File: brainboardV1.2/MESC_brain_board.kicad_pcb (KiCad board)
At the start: 4 copper layers, 64 x 84.5 mm, 52 parts, among them J1 Conn_01x18, J12 Conn_01x03, J13 Conn_01x03, J14 SERIAL1, J15 Conn_01x03, J21 Conn_01x07, J22 Conn_01x01, J24 Conn_01x01, J25 Conn_01x01, Q1 my_BC337, U1 TJA1050T/CM,118, U11 ESP32-WROOM-32D, U2 Teensy4.0, U21 LD1117S18TR_SOT223, U24 12_DCDC_5

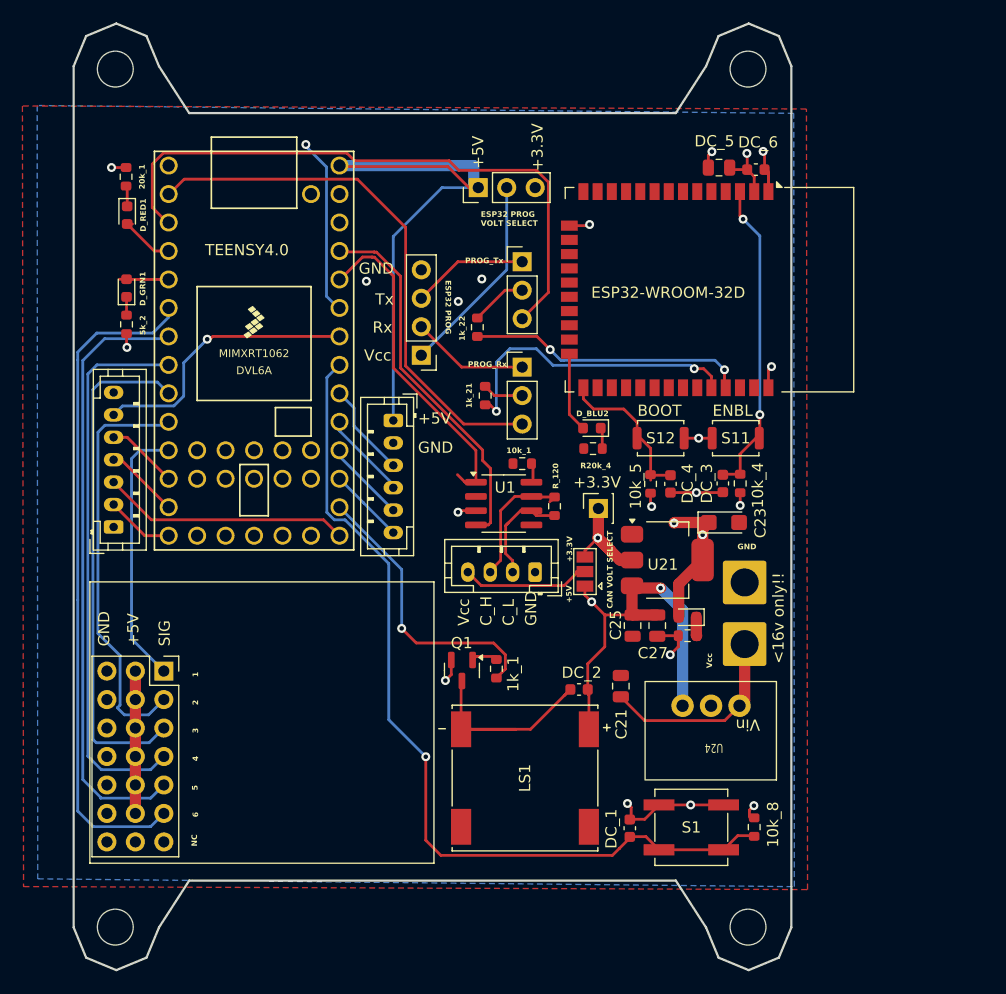
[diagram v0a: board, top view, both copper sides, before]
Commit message: documentation stuff
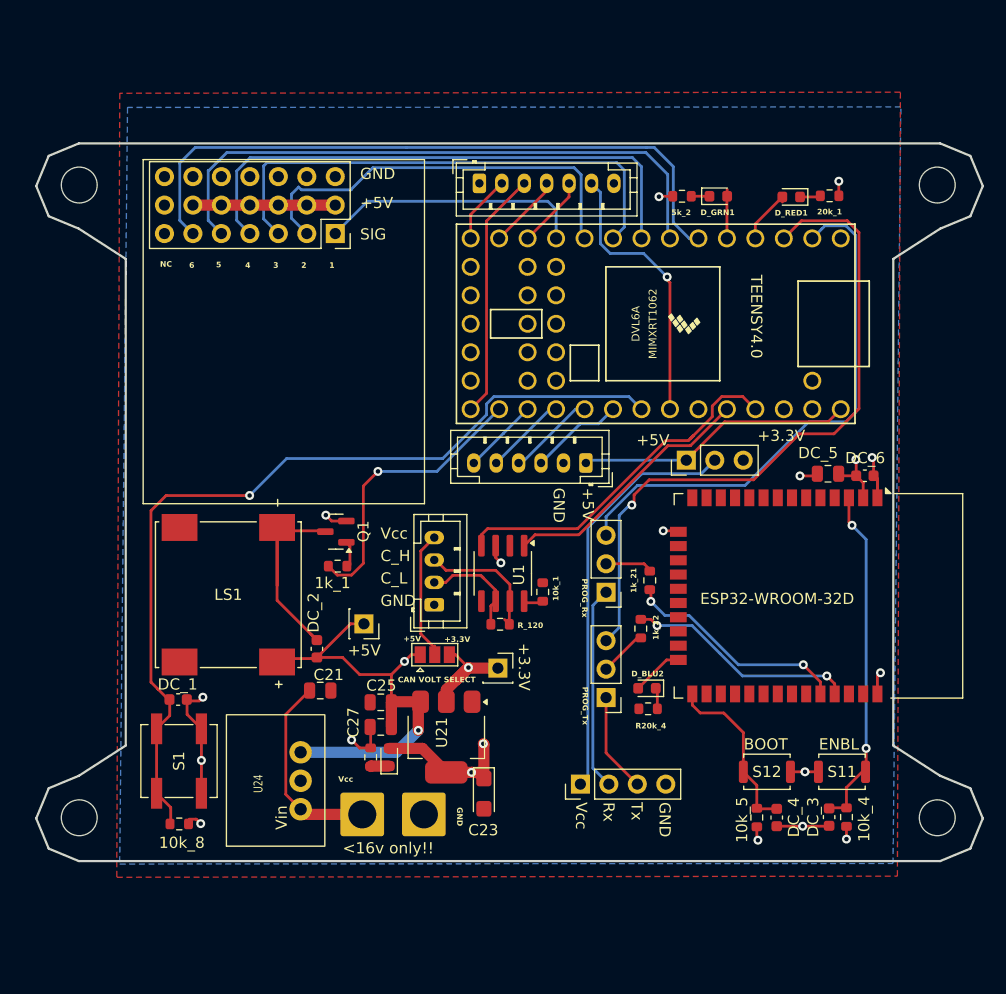
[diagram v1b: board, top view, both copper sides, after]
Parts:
- added J23: Conn_01x01, Connector_PinSocket_2.54mm:PinSocket_1x01_P2.54mm_Vertical, F.Cu at (45.5, 62.8)
- moved REF** 74.1 mm to (96.7, 23.7), turned to -90 degrees
- moved REF** 68.9 mm to (96.7, 80.1), turned to -90 degrees
- moved REF** 66.3 mm to (20.1, 23.7), turned to -90 degrees
- moved 20k_1 62.8 mm to (87.1, 24.7), turned to 180 degrees
- moved REF** 60.5 mm to (20.1, 80.1), turned to -90 degrees
- moved D_RED1 59.3 mm to (83.7, 24.8), turned to 180 degrees
- moved D_GRN1 53.4 mm to (77.1, 24.7), turned to 0 degrees
- moved 10k_8 51.3 mm to (29.1, 80.7), turned to 0 degrees
- moved 5k_2 50.9 mm to (73.9, 24.7), turned to 0 degrees
- moved S1 46.1 mm to (29.0, 75.1), turned to -90 degrees
- moved J21 44.8 mm to (55.8, 23.5), turned to 0 degrees
- moved J1 41.9 mm to (43.0, 28.0), turned to -90 degrees
- moved DC_1 41.9 mm to (29.0, 69.6), turned to 180 degrees
- moved J14 40.8 mm to (64.8, 77.1), turned to 90 degrees
- moved J13 39.6 mm to (67.1, 69.4), turned to 180 degrees
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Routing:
- net +5V: track 304.2 -> 278.2 mm
- net Net-(J14-Pin_1): track 18.1 -> 37.0 mm
- net unconnected-(U2-21_A7_RX5_BCLK1-Pad28): track 16.0 -> 0.00 mm, vias 1 -> 0
- net ESP_RX_OUT: track 10.5 -> 18.2 mm
- net U0RXD: track 27.6 -> 20.3 mm
- net /CAN_TX: track 29.8 -> 23.1 mm
- net ESP_TX: track 55.9 -> 61.0 mm, vias 0 -> 1
- net U0TXD: track 24.9 -> 20.7 mm
- net Net-(D_BLU2-A): track 7.14 -> 4.64 mm
- net ESP_EN: track 28.3 -> 30.6 mm
- net IO0: track 14.1 -> 15.6 mm
- net ESP_TX_OUT: track 10.4 -> 8.88 mm
- net /CAN_RX: track 33.1 -> 32.0 mm
- net Net-(J13-Pin_2): track 5.03 -> 4.26 mm
- net Net-(J12-Pin_2): track 3.64 -> 4.26 mm
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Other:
- board size 64 x 84.5 mm -> 84.5 x 64 mm
- board text removed: "ESP32 PROG"
- board text removed: "ESP32 PROG VOLT SELECT"
